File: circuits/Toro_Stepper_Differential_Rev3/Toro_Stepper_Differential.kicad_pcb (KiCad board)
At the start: 2 copper layers, 7 parts, among them J1 Screw_Terminal_01x03, J2 Screw_Terminal_01x02, J3 Screw_Terminal_01x03, J4 Screw_Terminal_01x02, U1 L293, U2 L293

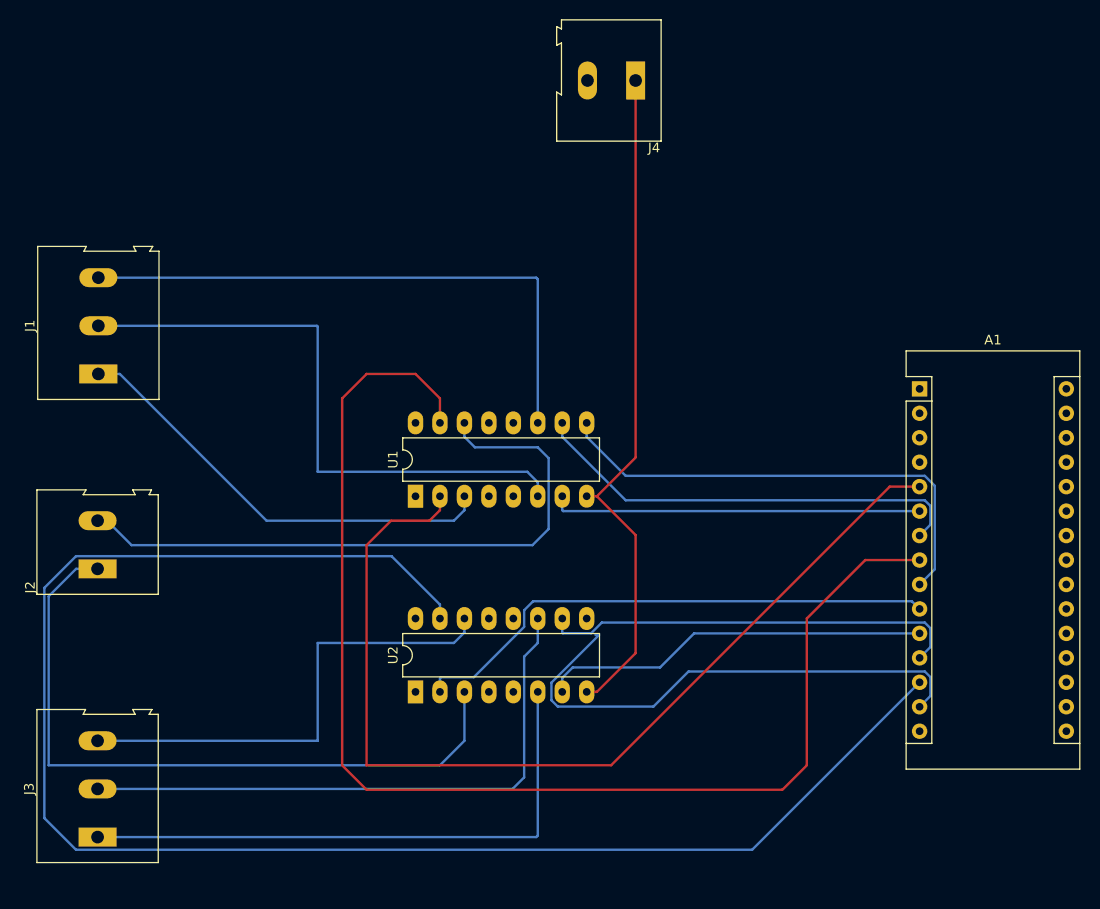
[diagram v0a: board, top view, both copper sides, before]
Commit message: updates
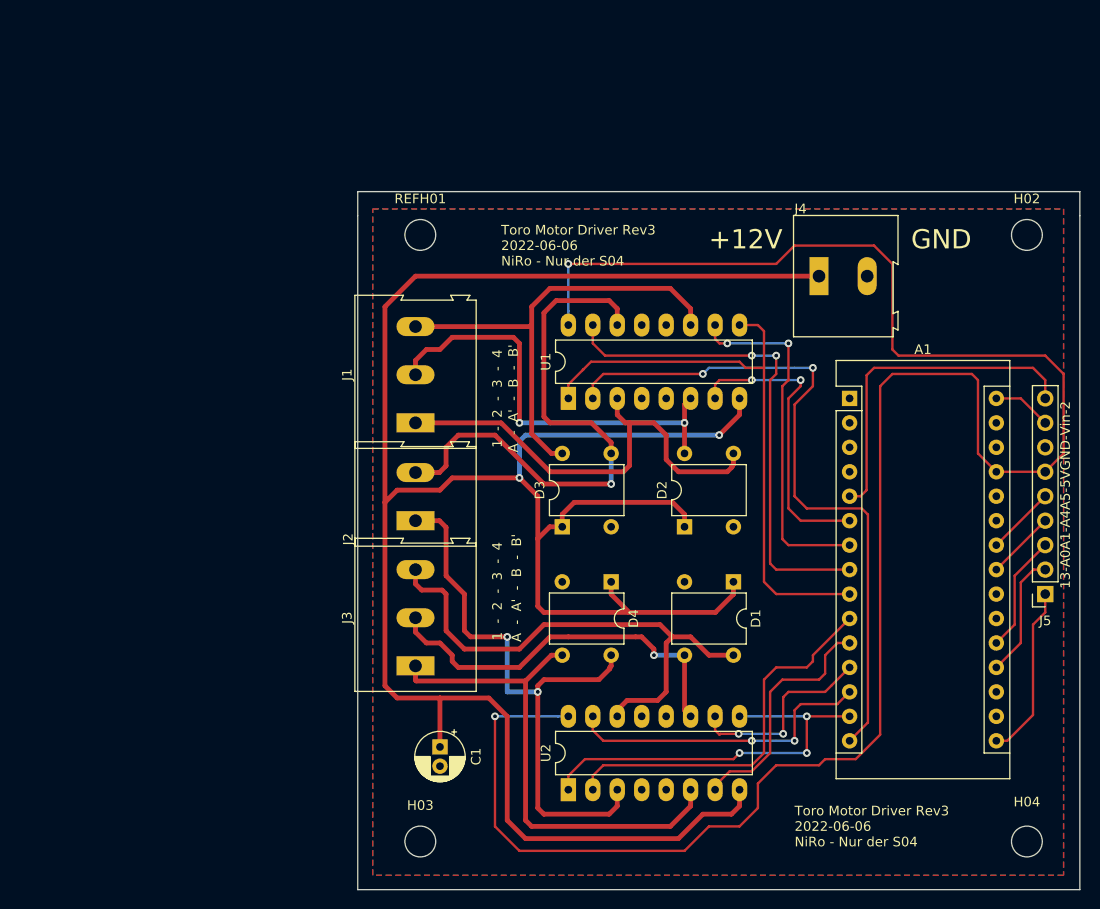
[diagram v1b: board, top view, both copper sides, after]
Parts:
- added C1: 220nF, Capacitor_THT:CP_Radial_D5.0mm_P2.00mm, F.Cu at (66.0, 130.2)
- added D1: D_Bridge_+-AA, nikos_footprints:BridgeRectifier_+-AA, F.Cu at (96.5, 113.0)
- added D2: D_Bridge_+-AA, nikos_footprints:BridgeRectifier_+-AA, F.Cu at (91.4, 107.3)
- added D3: D_Bridge_+-AA, nikos_footprints:BridgeRectifier_+-AA, F.Cu at (78.7, 107.3)
- added D4: D_Bridge_+-AA, nikos_footprints:BridgeRectifier_+-AA, F.Cu at (83.8, 113.0)
- added H02: MountingHole_3.2mm_M3_ISO14580, MountingHole:MountingHole_3.2mm_M3_ISO14580, F.Cu at (127.0, 77.0)
- added H03: MountingHole_3.2mm_M3_ISO14580, MountingHole:MountingHole_3.2mm_M3_ISO14580, F.Cu at (64.0, 140.0)
- added H04: MountingHole_3.2mm_M3_ISO14580, MountingHole:MountingHole_3.2mm_M3_ISO14580, F.Cu at (127.0, 140.0)
- added J5: Conn_01x09_Male, Connector_PinSocket_2.54mm:PinSocket_1x09_P2.54mm_Vertical, F.Cu at (128.9, 114.3)
- added REFH01: MountingHole_3.2mm_M3_ISO14580, MountingHole:MountingHole_3.2mm_M3_ISO14580, F.Cu at (64.0, 77.0)
- J4: value Screw_Terminal_01x02 -> Screw_Terminal _01x02
- moved J3 37.5 mm to (63.5, 121.8)
- moved J2 33.4 mm to (63.5, 106.7)
- moved J1 33.3 mm to (63.5, 96.5)
- moved J4 27.9 mm to (105.4, 81.3), turned to 0 degrees
- moved U2 18.8 mm to (79.4, 134.6)
- moved U1 18.8 mm to (79.4, 94.0)
- moved A1 7.34 mm to (108.6, 94.0)
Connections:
- U1 pad 2: Net-(A1-Pad5) -> Net-(A1-Pad15)
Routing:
- net Net-(A1-Pad27): track 0.00 -> 209.4 mm, vias 0 -> 2
- net +10V: track 70.6 -> 248.4 mm, vias 0 -> 2
- net Net-(A1-Pad13): track 169.4 -> 32.5 mm, vias 0 -> 2
- net Net-(A1-Pad8): track 132.7 -> 51.9 mm, vias 0 -> 2
- net Net-(A1-Pad15): track 0.00 -> 71.8 mm, vias 0 -> 2
- net Net-(A1-Pad5): track 102.9 -> 35.3 mm
- net Net-(A1-Pad12): track 44.0 -> 20.7 mm, vias 0 -> 2
- net Net-(D1-Pad3): track 61.9 -> 40.4 mm, vias 0 -> 1
- net Net-(A1-Pad16): track 0.00 -> 18.0 mm
- net Net-(D2-Pad4): track 62.7 -> 44.9 mm, vias 0 -> 2
- net Net-(A1-Pad10): track 55.9 -> 39.7 mm
- net Net-(A1-Pad11): track 40.5 -> 25.4 mm
- net Net-(A1-Pad19): track 0.00 -> 13.0 mm
- net Net-(A1-Pad20): track 0.00 -> 12.3 mm
- net Net-(A1-Pad14): track 54.1 -> 42.4 mm, vias 0 -> 3
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- added copper zone on F.Cu, net +10V
- added copper zone on B.Cu, net GND
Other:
- board outline added: 75 x 72.5 mm
- board text added: "+12V"
- board text added: "1 - 2 - 3 - 4"
- board text added: "13-A0A1-A4A5-5VGND-Vin-2"
- board text added: "A - A' - B - B'"
- board text added: "GND"
- board text added: "Toro Motor Driver Rev3 2022-06-06 NiRo - Nur der S04"
